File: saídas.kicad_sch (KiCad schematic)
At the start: 36 parts, among them J10 CARGA_12V, J12 Habilita buzzer, J13 Habilita rele, J6 MOTOR, J7 PWM_SERVO, J8 PWM_SERVO, J9 Screw_Terminal_01x03, K1 Relay_SPDT_Latching_1coil, Q1 2N7002, Q2 SI4483ADY-T1-GE3, Q3 2N7002, Q4 2N7002, U6 AS4950

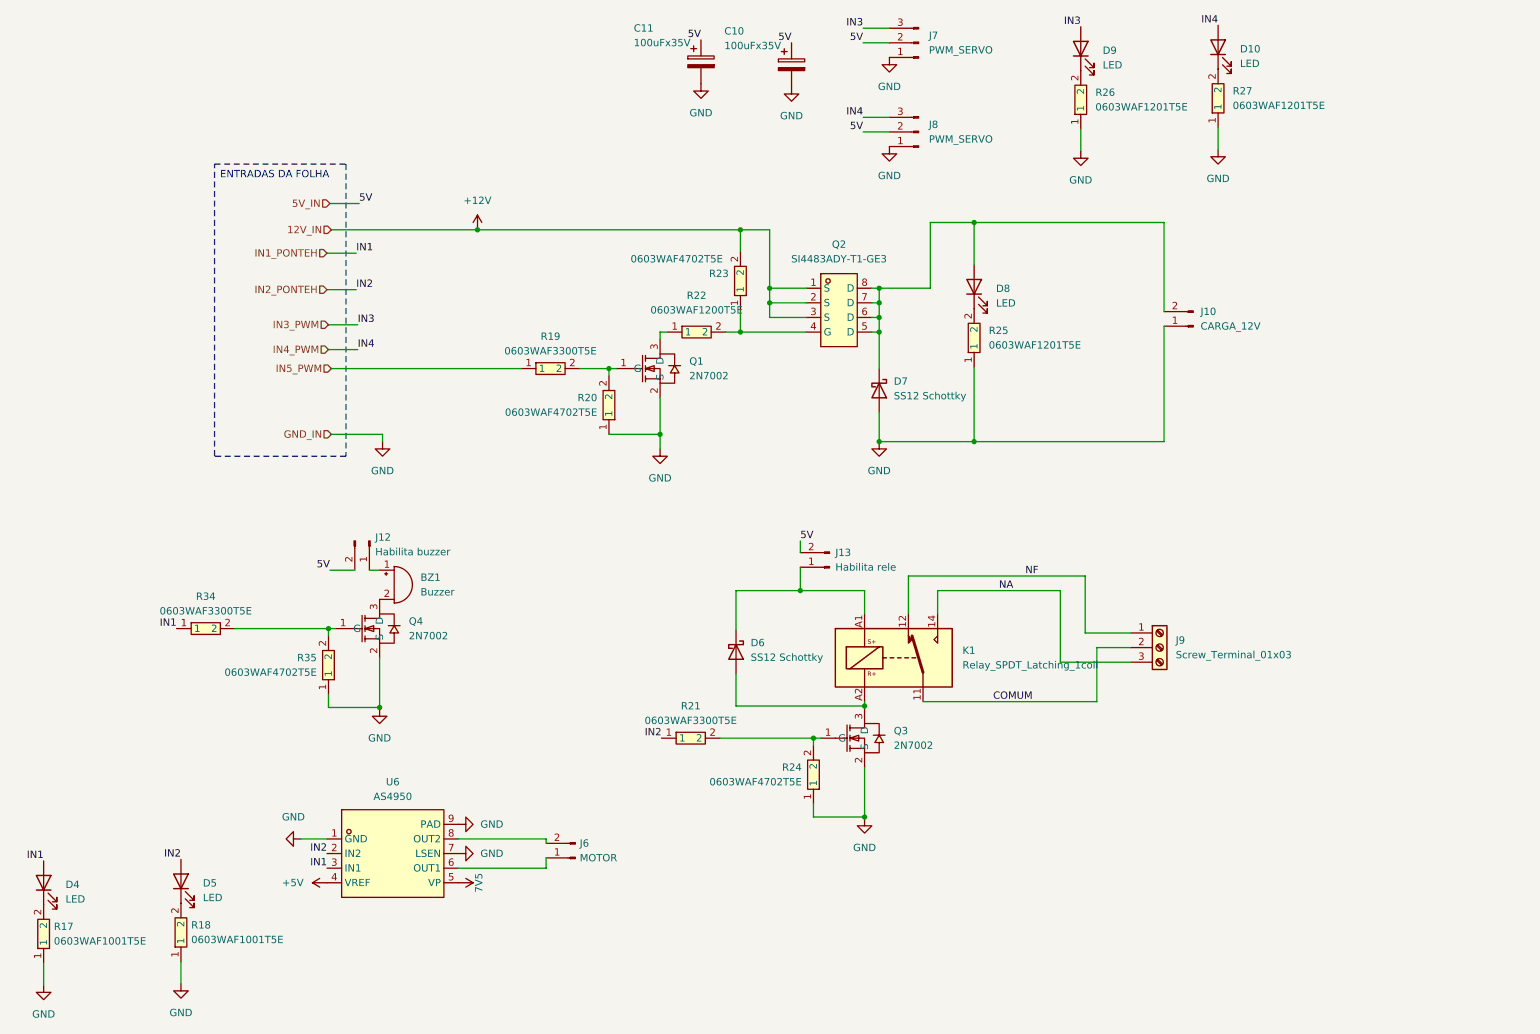
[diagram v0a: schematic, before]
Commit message: organização e legendas do esquemático
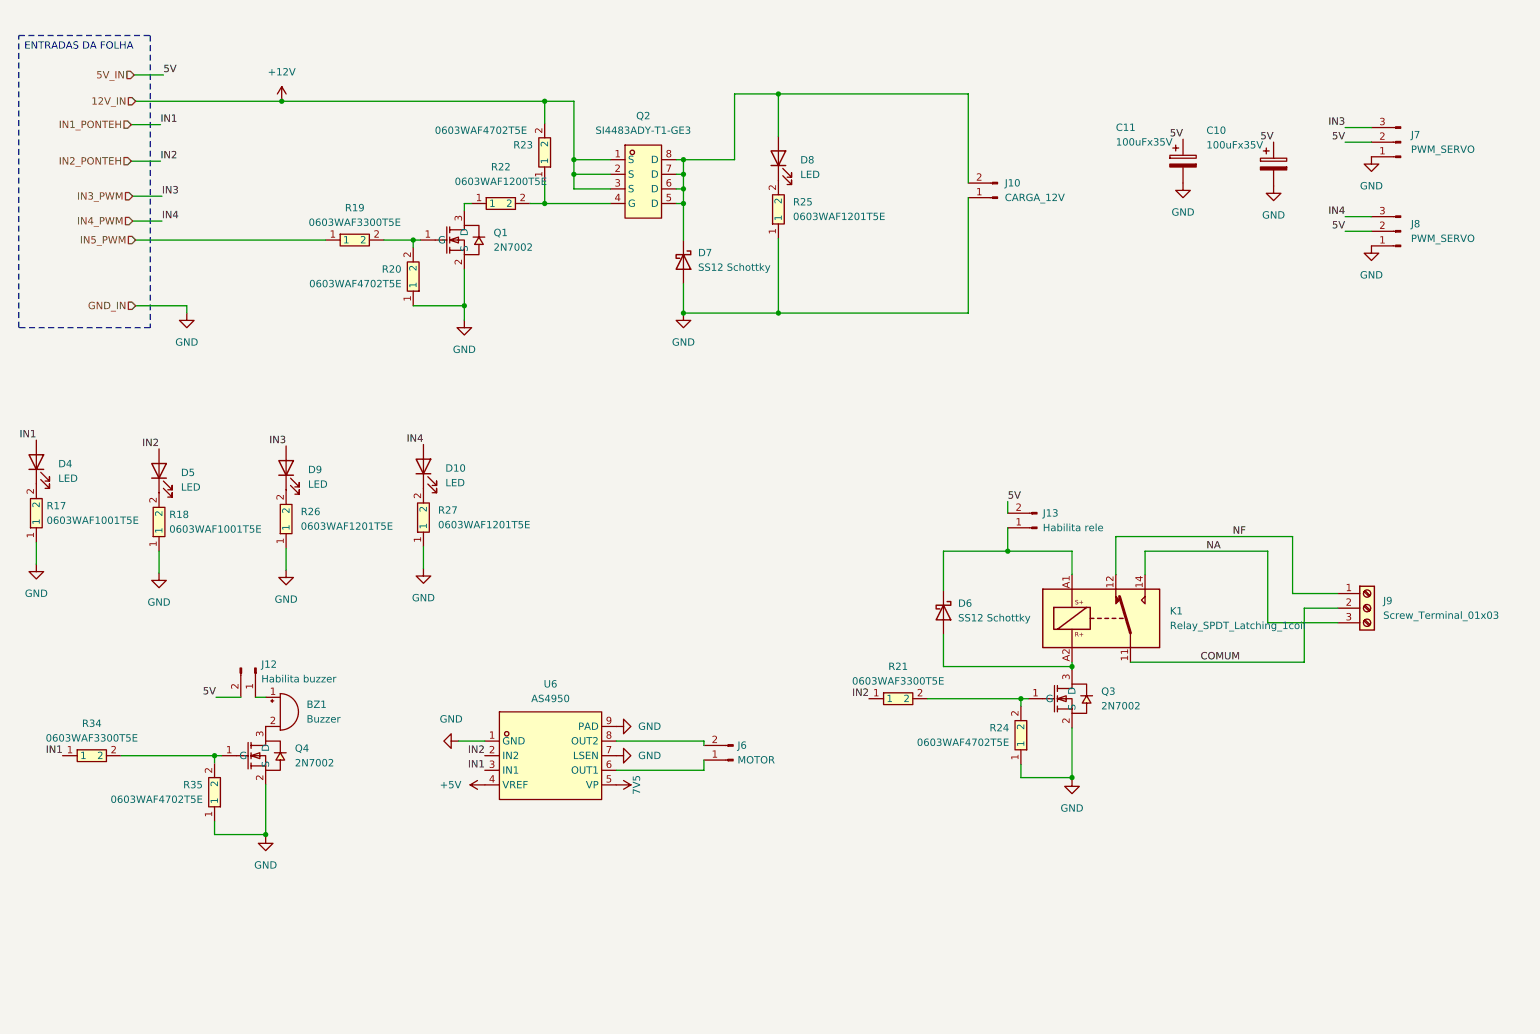
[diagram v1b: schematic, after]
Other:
- moved on the sheet: BZ1, C10, C11, D10, D4, D5, D6, D7, D8, D9, J10, J12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
